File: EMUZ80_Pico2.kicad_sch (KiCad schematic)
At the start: 16 parts, among them J1 Conn_01x20_Socket, J2 Conn_01x20_Socket, SW1 SW_Push, SW2 SW_Push, U1 Pimoroni PGA2350B, U2 RB2350B_Core_Board, U3 74HC00, U4 Z80CPU, U5 HM628128_DIP32_SOP32

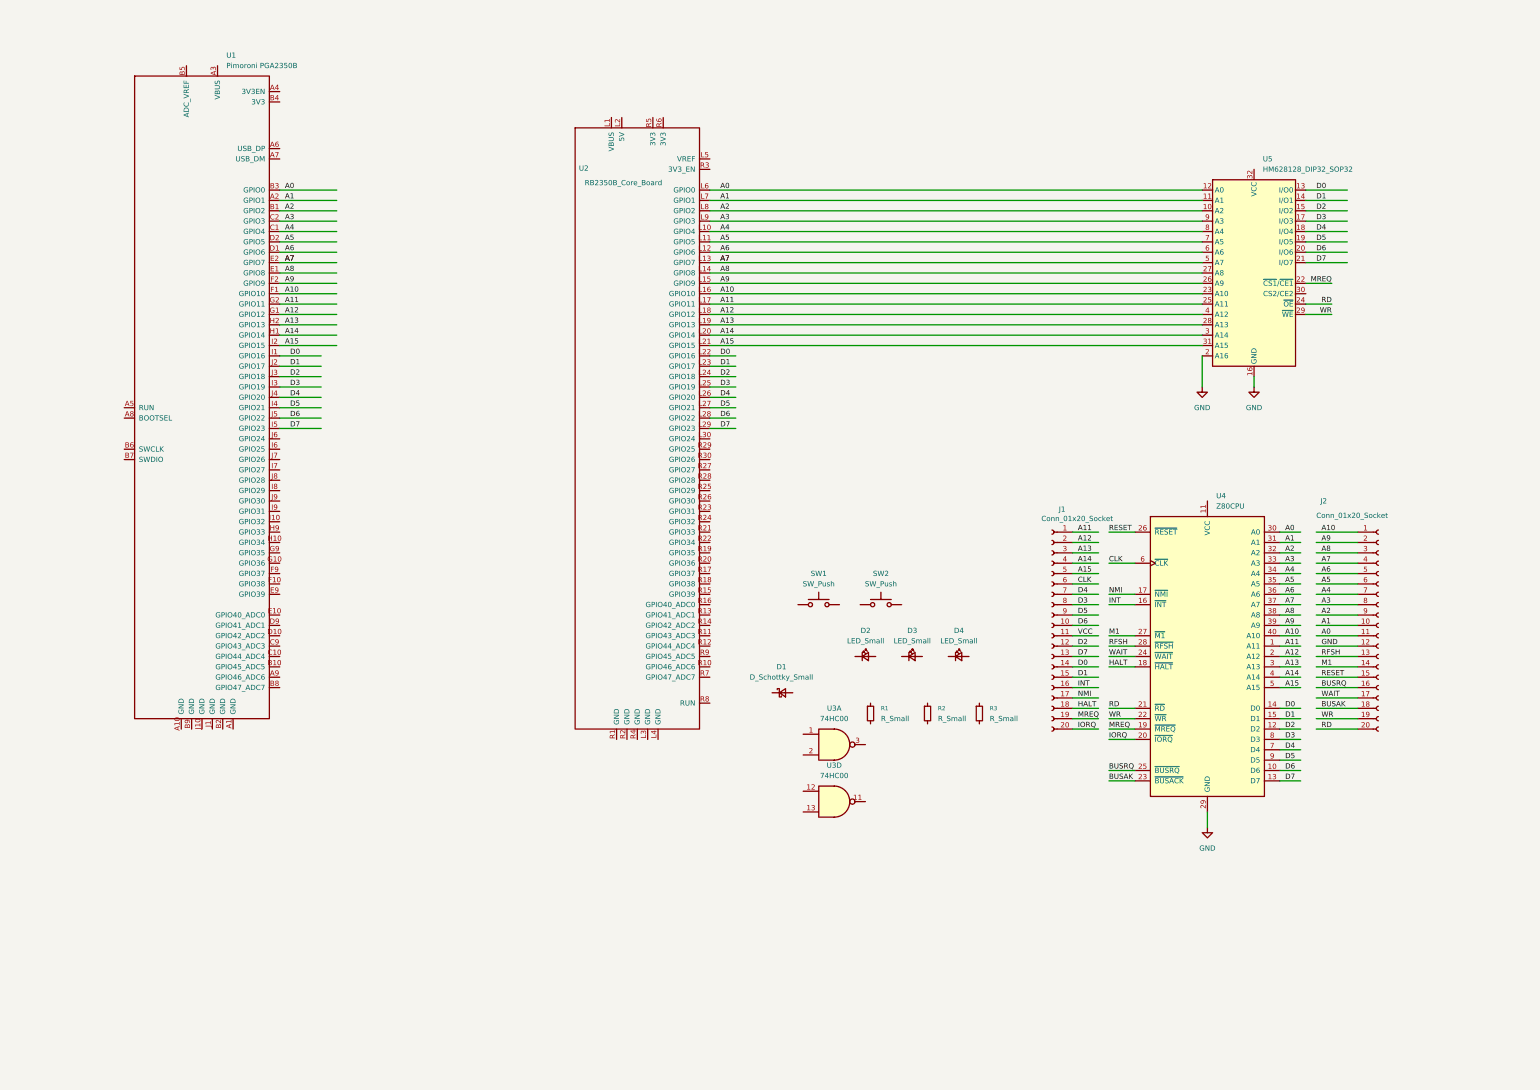
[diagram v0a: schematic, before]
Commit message: schematic finished
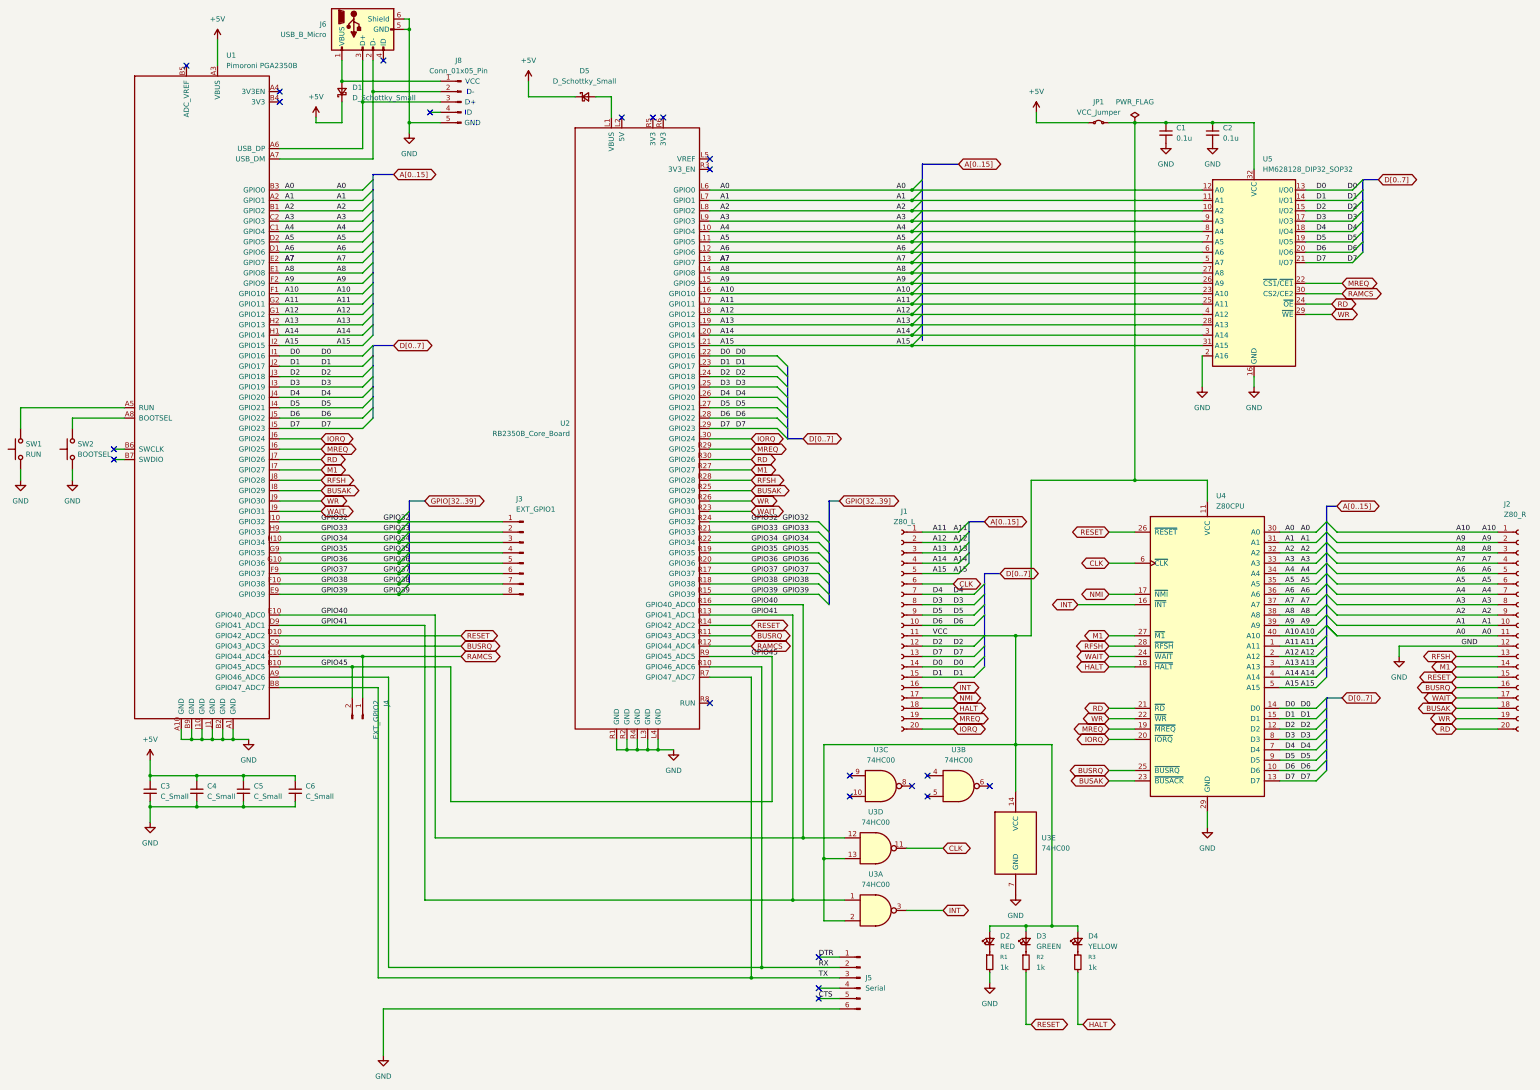
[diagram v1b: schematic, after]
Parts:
- removed J1, J2: Conn_01x20_Socket, Connector_PinSocket_2.54mm:PinSocket_1x20_P2.54mm_Vertical, symbol kuma-lib1:Conn_01x20_Socket
- removed U3: 74HC00, Package_DIP:DIP-14_W7.62mm_Socket, symbol kuma-lib1:74HC00
- added C1, C2: 0.1u, symbol Device:C_Small
- added C3, C4, C5, C6: C_Small, symbol Device:C_Small
- added D5: D_Schottky_Small, symbol local:D_Schottky_Small
- added J1: Z80_L, symbol local:Conn_01x20_Socket
- added J2: Z80_R, symbol local:Conn_01x20_Socket
- added J3: EXT_GPIO1, symbol Connector:Conn_01x08_Pin
- added J4: EXT_GPIO2, symbol Connector:Conn_01x02_Pin
- added J5: Serial, symbol Connector:Conn_01x06_Pin
- added J6: USB_B_Micro, symbol Connector:USB_B_Micro
- added J8: Conn_01x05_Pin, symbol Connector:Conn_01x05_Pin
- added JP1: VCC_Jumper, symbol Jumper:Jumper_2_Small_Bridged
- added U3: 74HC00, symbol local:74HC00
- D2: value LED_Small -> RED; footprint kuma-f:LED_D3.0mm -> local-f:LED_D3.0mm
- D3: value LED_Small -> GREEN; footprint kuma-f:LED_D3.0mm -> local-f:LED_D3.0mm
- D4: value LED_Small -> YELLOW; footprint kuma-f:LED_D3.0mm -> local-f:LED_D3.0mm
- R1, R2, R3: value R_Small -> 1k; footprint kuma-f:R_Axial_DIN0207_L6.3mm_D2.5mm_P7.62mm_Horizontal -> local-f:R_Axial_DIN0207_L6.3mm_D2.5mm_P7.62mm_Horizontal
- SW1: value SW_Push -> RUN; footprint kuma-f:Tact_SW -> local-f:Tact_SW
- SW2: value SW_Push -> BOOTSEL; footprint kuma-f:Tact_SW -> local-f:Tact_SW
- U2: footprint local-f:RB2350B_Core_Board -> (none)
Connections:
- net A0: now also J2.11 (Pin_11)
- net A1: now also J2.10 (Pin_10)
- net A10: now also J2.1 (Pin_1)
- net A11: now also J1.1 (Pin_1)
- net A12: now also J1.2 (Pin_2)
- net A13: now also J1.3 (Pin_3)
- net A14: now also J1.4 (Pin_4)
- net A15: now also J1.5 (Pin_5)
- net A2: now also J2.9 (Pin_9)
- net A3: now also J2.8 (Pin_8)
- net A4: now also J2.7 (Pin_7)
- net A5: now also J2.6 (Pin_6)
- net A6: now also J2.5 (Pin_5)
- net A7: now also J2.4 (Pin_4)
- net A8: now also J2.3 (Pin_3)
- net A9: now also J2.2 (Pin_2)
- net BUSAK: now also U1.I8 (GPIO29), U2.R25 (GPIO29), J2.18 (Pin_18)
- net BUSRQ: now also U1.C9 (GPIO43_ADC3), U2.R11 (GPIO43_ADC3), J2.16 (Pin_16)
- net CLK: now also J1.6 (Pin_6), U3.11
- net D0: now also J1.14 (Pin_14)
- net D1: now also J1.15 (Pin_15)
- net D2: now also J1.12 (Pin_12)
- net D3: now also J1.8 (Pin_8)
- net D4: now also J1.7 (Pin_7)
- net D5: now also J1.9 (Pin_9)
- net D6: now also J1.10 (Pin_10)
- net D7: now also J1.13 (Pin_13)
- net GND: now also R1.2, SW1.1, SW2.1, U1.A1 (GND), U1.A10 (GND), U1.B2 (GND), U1.B9 (GND), U1.J1 (GND), U1.J10 (GND), U2.L3 (GND), U2.L4 (GND), U2.R1 (GND), U2.R2 (GND), U2.R4 (GND), C1.2, C2.2, C3.2, C4.2, C5.2, C6.2, J2.12 (Pin_12), J5.6 (Pin_6), J6.5 (GND), J6.6 (Shield), J8.5 (Pin_5), U3.7 (GND)
- net HALT: now also R3.2, J1.18 (Pin_18)
- net INT: now also J1.16 (Pin_16), U3.3
- net IORQ: now also U1.J6 (GPIO24), U2.L30 (GPIO24), J1.20 (Pin_20)
- net M1: now also U1.I7 (GPIO27), U2.R27 (GPIO27), J2.14 (Pin_14)
- net MREQ: now also U1.I6 (GPIO25), U2.R29 (GPIO25), J1.19 (Pin_19)
- net NMI: now also J1.17 (Pin_17)
- net RD: now also U1.J7 (GPIO26), U2.R30 (GPIO26), J2.20 (Pin_20)
- net RESET: now also R2.2, U1.D10 (GPIO42_ADC2), U2.R14 (GPIO42_ADC2), J2.15 (Pin_15)
- net RFSH: now also U1.J8 (GPIO28), U2.R28 (GPIO28), J2.13 (Pin_13)
- net VCC: now also D2.2 (A), D3.2 (A), D4.2 (A), U4.11 (VCC), U5.32 (VCC), C1.1, C2.1, J1.11 (Pin_11), JP1.2 (B), U3.13, U3.14 (VCC), U3.2
- net WAIT: now also U1.I9 (GPIO31), U2.R23 (GPIO31), J2.17 (Pin_17)
- net WR: now also U1.J9 (GPIO30), U2.R26 (GPIO30), J2.19 (Pin_19)
- net +5V: now reaches D1.1 (K)
- net +5V: now also U1.A3 (VBUS), C3.1, C4.1, C5.1, C6.1, D5.1 (K), JP1.1 (A)
- net at D1.2 (A): now also J6.1 (VBUS), J8.1 (Pin_1)
- net at D3.1 (K): now also R2.1
- net at R1.1: now also D2.1 (K)
- net RAMCS: now reaches U5.30 (CS2/CE2)
- net RAMCS: now also U1.C10 (GPIO44_ADC4), U2.R12 (GPIO44_ADC4), J4.1 (Pin_1)
- net at D4.1 (K): now also R3.1
- net at U2.L1 (VBUS): now also D5.2 (A)
- net RX: now reaches U2.R10 (GPIO46_ADC6)
- net RX: now also U1.A9 (GPIO46_ADC6), J5.2 (Pin_2)
- net GPIO41: now reaches U2.R13 (GPIO41_ADC1)
- net GPIO41: now also U1.D9 (GPIO41_ADC1), U3.1
- net GPIO39: now reaches U2.R15 (GPIO39)
- net GPIO39: now also U1.E9 (GPIO39), J3.8 (Pin_8)
- net GPIO40: now reaches U2.R16 (GPIO40_ADC0)
- net GPIO40: now also U1.E10 (GPIO40_ADC0), U3.12
- net GPIO37: now reaches U2.R17 (GPIO37)
- net GPIO37: now also U1.F9 (GPIO37), J3.6 (Pin_6)
- net GPIO38: now reaches U2.R18 (GPIO38)
- net GPIO38: now also U1.F10 (GPIO38), J3.7 (Pin_7)
- net GPIO35: now reaches U2.R19 (GPIO35)
- net GPIO35: now also U1.G9 (GPIO35), J3.4 (Pin_4)
- net GPIO36: now reaches U2.R20 (GPIO36)
- net GPIO36: now also U1.G10 (GPIO36), J3.5 (Pin_5)
- net GPIO33: now reaches U2.R21 (GPIO33)
- net GPIO33: now also U1.H9 (GPIO33), J3.2 (Pin_2)
- net GPIO34: now reaches U2.R22 (GPIO34)
- net GPIO34: now also U1.H10 (GPIO34), J3.3 (Pin_3)
- net GPIO32: now reaches U2.R24 (GPIO32)
- net GPIO32: now also U1.I10 (GPIO32), J3.1 (Pin_1)
- net TX: now reaches U2.R7 (GPIO47_ADC7)
- net TX: now also U1.B8 (GPIO47_ADC7), J5.3 (Pin_3)
- net GPIO45: now reaches U2.R9 (GPIO45_ADC5)
- net GPIO45: now also U1.B10 (GPIO45_ADC5), J4.2 (Pin_2)
- net at U1.A5 (RUN): now also SW1.2
- net at U1.A6 (USB_DP): now also J6.3 (D+), J8.3 (Pin_3)
- net at U1.A7 (USB_DM): now also J6.2 (D-), J8.2 (Pin_2)
- net at U1.A8 (BOOTSEL): now also SW2.2
- new net CTS: J5.5 (Pin_5)
- new net DTR: J5.1 (Pin_1)
- no-connect marks 0 -> 22
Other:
- note added: "D+"
- note added: "D-"
- note added: "GND"
- note added: "ID"
- note added: "VCC"
- moved on the sheet: D1, D2, D3, D4, R1, R2, R3, SW1, SW2
